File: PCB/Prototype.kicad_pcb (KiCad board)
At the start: 2 copper layers, 38.1 x 59.5 mm, 7 parts, among them SW5 SW_Push, SW6 SW_Push, SW7 SW_Push, SW8 SW_Push, U1 XIAO-RP2040-DIP

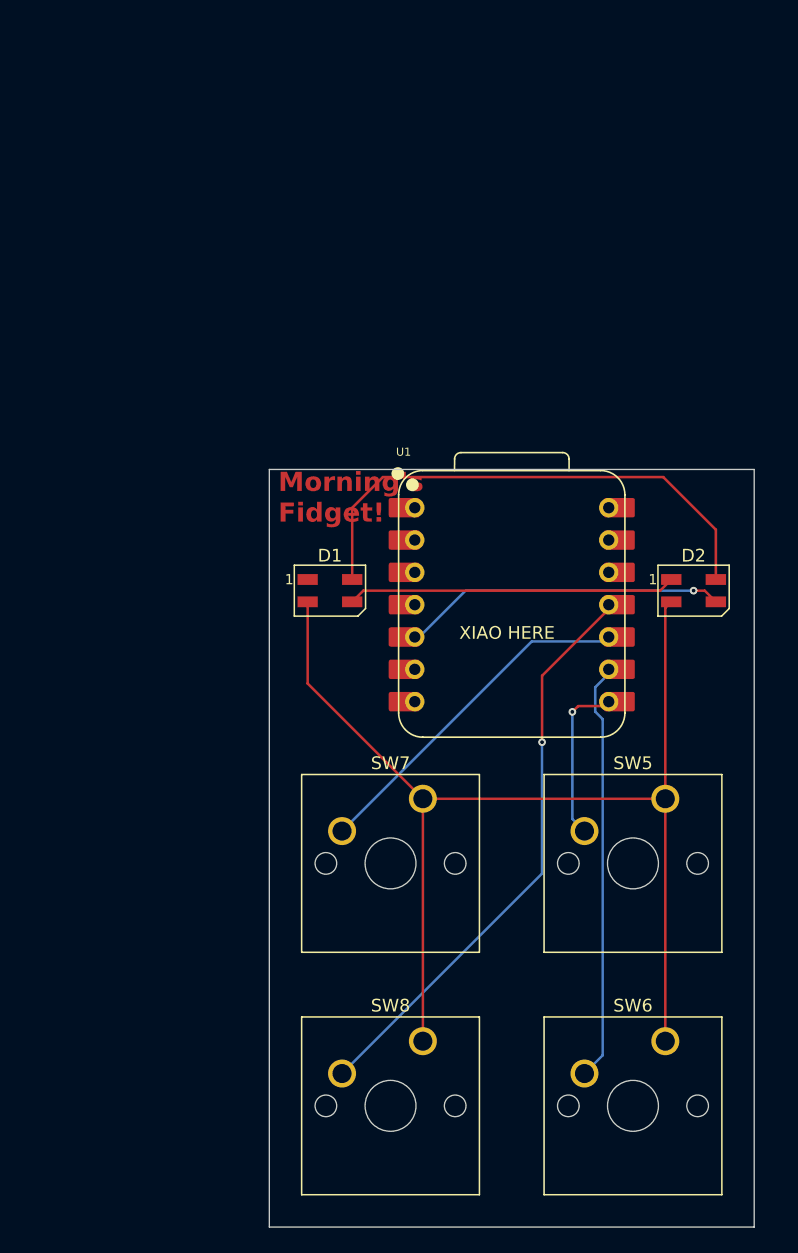
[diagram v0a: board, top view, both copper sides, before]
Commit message: Initial commit!!
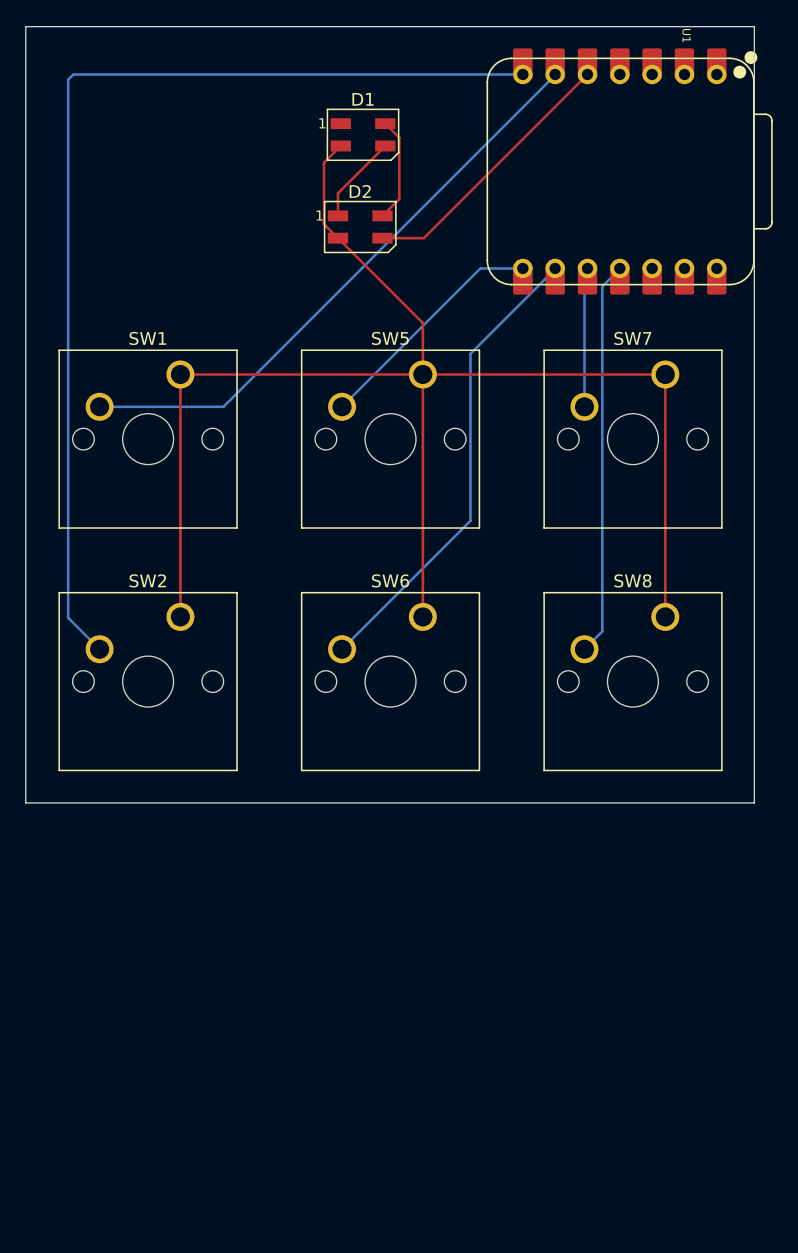
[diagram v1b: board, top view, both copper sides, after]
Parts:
- added SW1: SW_Push, Button_Switch_Keyboard:SW_Cherry_MX_1.00u_PCB, F.Cu at (140.7, 56.8)
- added SW2: SW_Push, Button_Switch_Keyboard:SW_Cherry_MX_1.00u_PCB, F.Cu at (140.7, 75.9)
- moved D2 38.8 mm to (154.8, 45.2)
- moved SW5 38.4 mm to (159.7, 56.8)
- moved SW6 38.4 mm to (159.7, 75.9)
- moved SW7 38.4 mm to (178.8, 56.8)
- moved SW8 38.4 mm to (178.8, 75.9)
- moved D1 35.9 mm to (155.0, 38.0)
- moved U1 35.1 mm to (175.2, 40.9), turned to -90 degrees
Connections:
- U1 pad 6: unconnected-(U1-GPIO7/SCL-Pad6) -> Net-(U1-GPIO7/SCL)
- U1 pad 7: unconnected-(U1-GPIO0/TX-Pad7) -> Net-(U1-GPIO0/TX)
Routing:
- net Net-(U1-GPIO0/TX): track 0.00 -> 81.7 mm
- net Net-(U1-GPIO7/SCL): track 0.00 -> 46.7 mm
- net +5V: track 40.8 -> 8.25 mm
- net GND: track 92.0 -> 117.0 mm
- net Net-(D1-DIN): track 25.8 -> 7.03 mm
- net Net-(U1-GPIO4/MISO): track 27.1 -> 11.0 mm
- net Net-(U1-GPIO3/MOSI): track 45.2 -> 31.1 mm, vias 1 -> 0
- net Net-(U1-GPIO1/RX): track 12.8 -> 18.8 mm, vias 1 -> 0
- net Net-(D2-DIN): track 25.7 -> 21.4 mm, vias 1 -> 0
- net Net-(U1-GPIO2/SCK): track 32.7 -> 36.9 mm
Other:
- board size 38.1 x 59.5 mm -> 57.2 x 61 mm
- board text removed: "Morning's Fidget!"
- board text removed: "XIAO HERE"
